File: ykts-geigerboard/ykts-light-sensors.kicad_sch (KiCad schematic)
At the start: 26 parts, among them J91 LSENSE_X+, J92 LSENSE_X-, J93 LSENSE_Y+, J94 LSENSE_Y-, J95 LSENSE_Z+, J96 LSENSE_Z-, Q1 RJU003N03 NMOS, Q2 RJU003N03 NMOS, U6 ATmega328P-AU, Y1 8 MHz

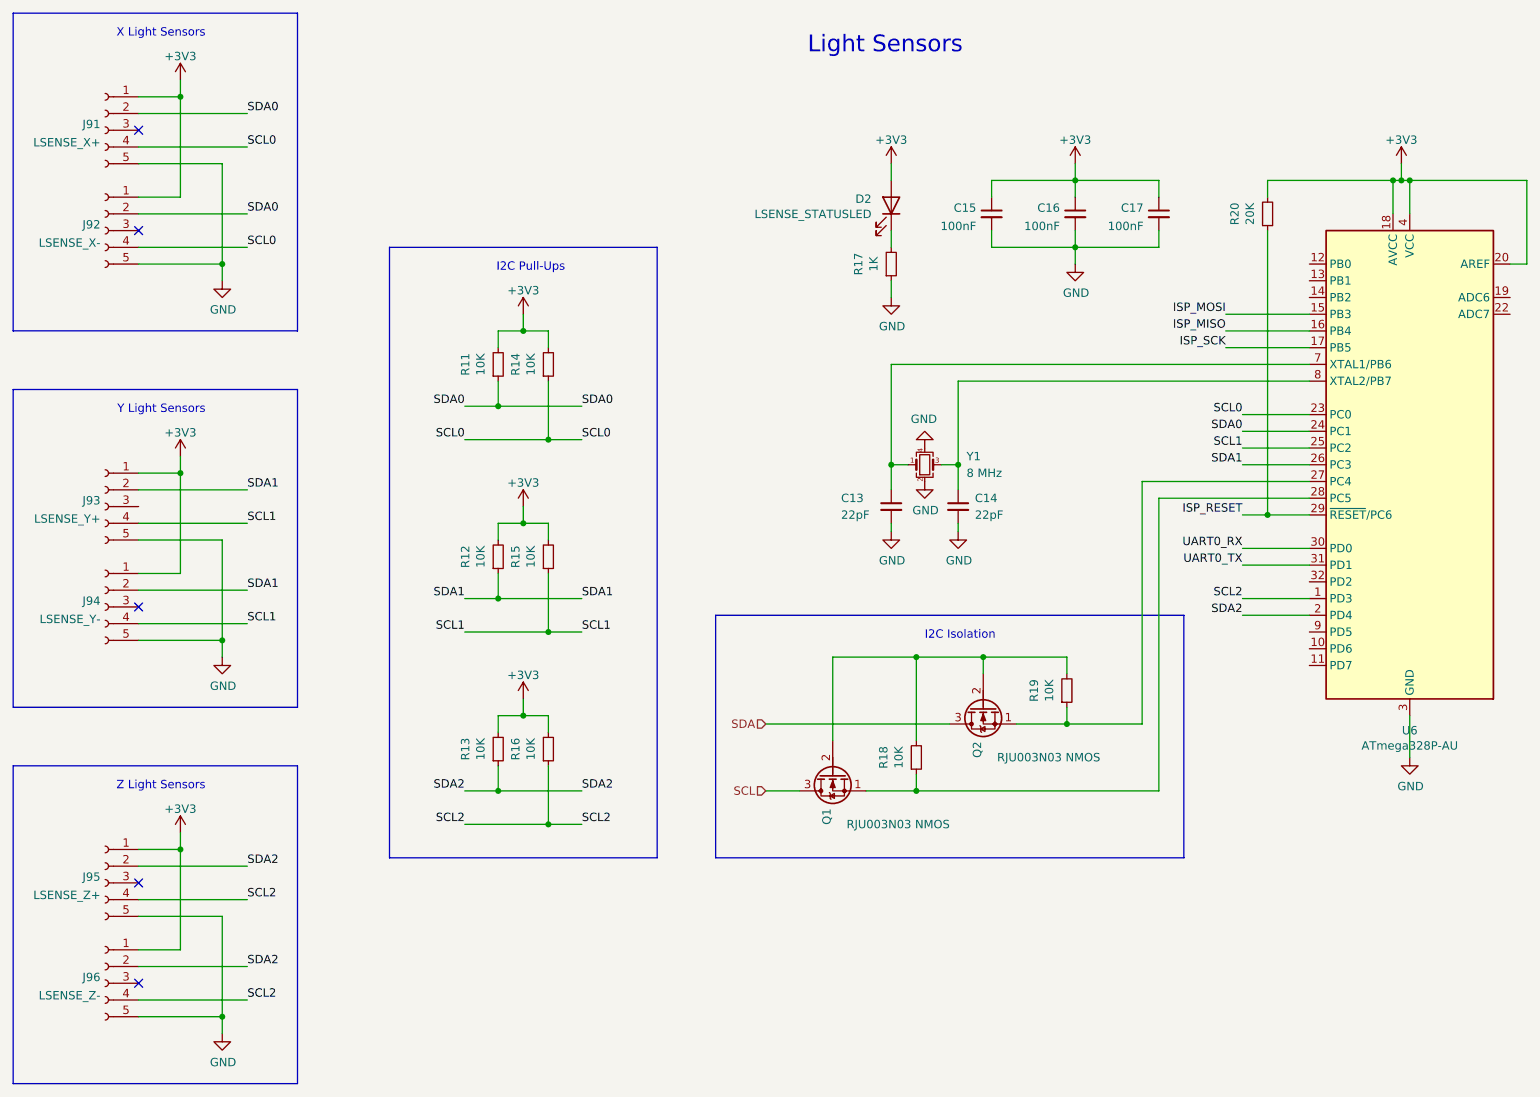
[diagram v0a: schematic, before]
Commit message: Sync with remote
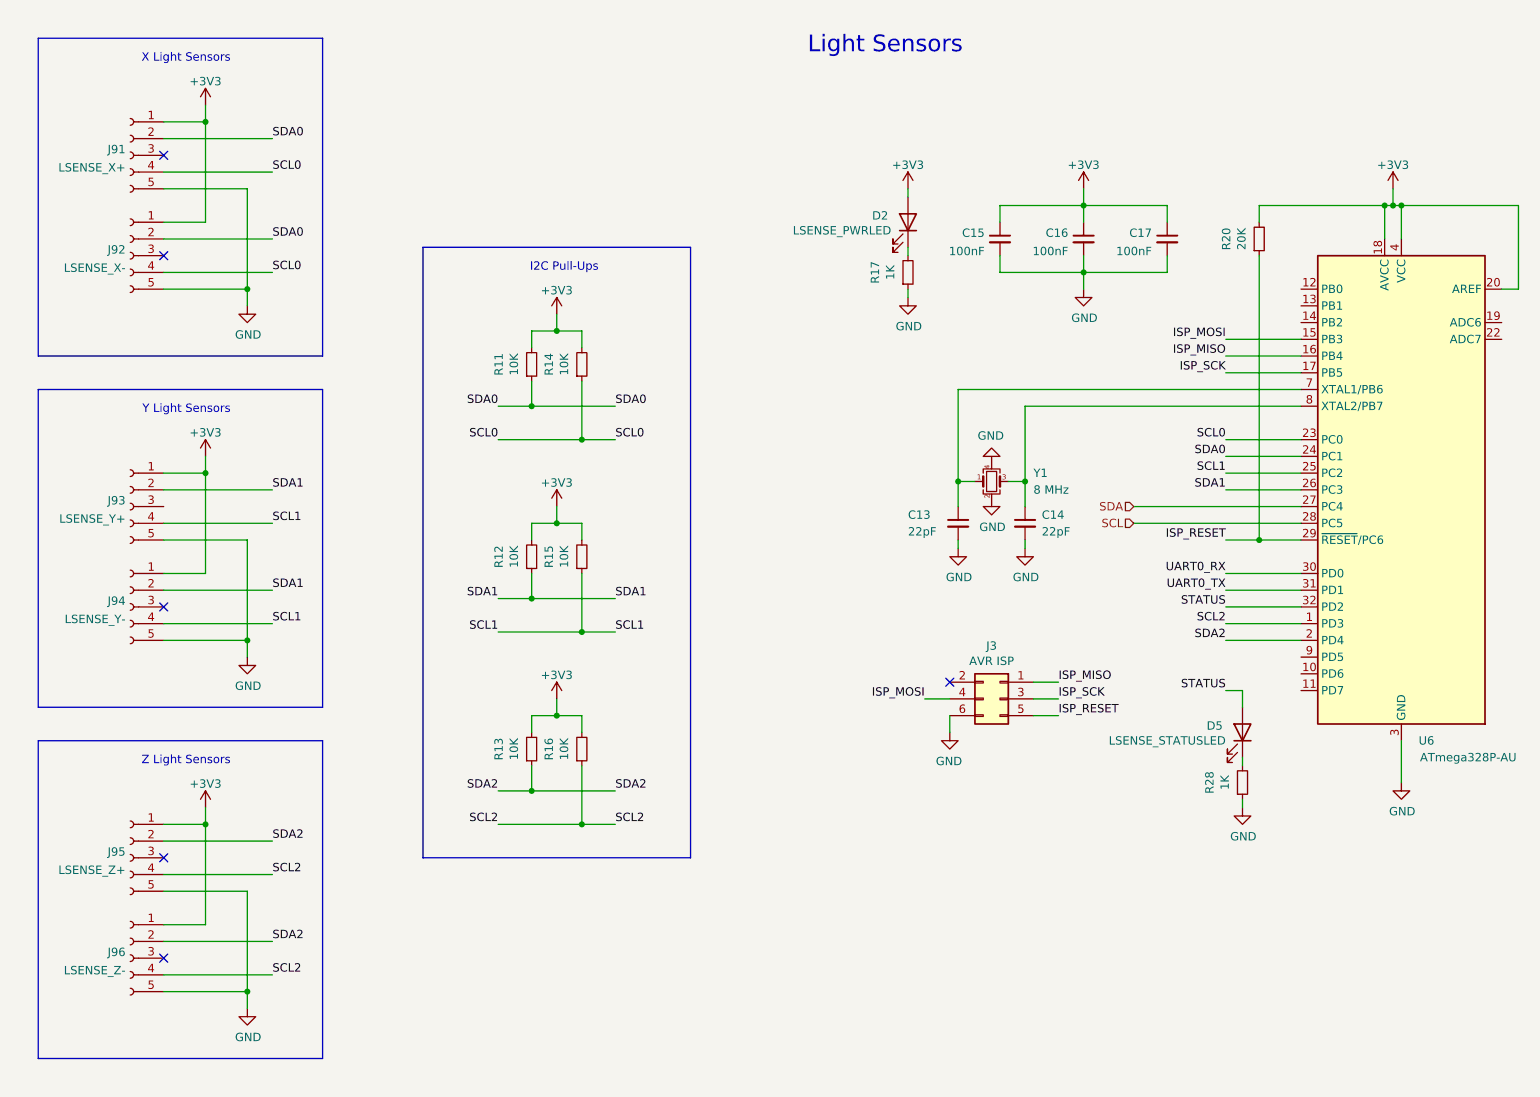
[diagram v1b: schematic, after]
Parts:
- removed Q1, Q2: RJU003N03 NMOS, Package_TO_SOT_SMD:SOT-323_SC-70, symbol Device:Q_NMOS_SGD
- removed R18, R19: 10K, Resistor_SMD:R_0402_1005Metric, symbol Device:R_Small
- added D5: LSENSE_STATUSLED, LED_SMD:LED_0402_1005Metric, symbol Device:LED
- added J3: AVR ISP, Connector_PinHeader_1.27mm:PinHeader_2x03_P1.27mm_Vertical_SMD, symbol Connector_Generic:Conn_02x03_Odd_Even
- added R28: 1K, Resistor_SMD:R_0402_1005Metric, symbol Device:R_Small
- D2: value LSENSE_STATUSLED -> LSENSE_PWRLED
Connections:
- net GND: now also J3.6 (Pin_6), R28.1
- net ISP_MISO: now also J3.1 (Pin_1)
- net ISP_MOSI: now also J3.4 (Pin_4)
- net ISP_RESET: now also J3.5 (Pin_5)
- net ISP_SCK: now also J3.3 (Pin_3)
- net SCL: now also U6.28 (PC5)
- net SDA: now also U6.27 (PC4)
- net STATUS: now reaches U6.32 (PD2)
- net STATUS: now also D5.2 (A)
- new net: D5.1 (K), R28.2
- no-connect marks 5 -> 6
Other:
- note removed: "I2C Isolation"
- moved on the sheet: C13, C14, C15, C16, C17, D2, J91, J92, J93, J94, J95, J96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
